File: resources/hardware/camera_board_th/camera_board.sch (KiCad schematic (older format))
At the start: 10 parts, among them P1 CONN_01X03, Q1 Q_NPN_EBC

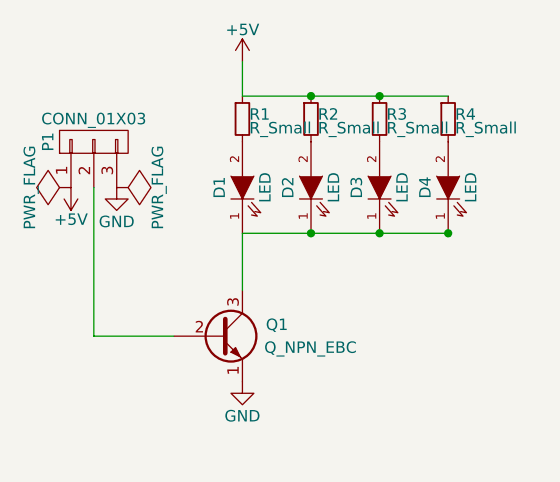
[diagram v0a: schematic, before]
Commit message: nt
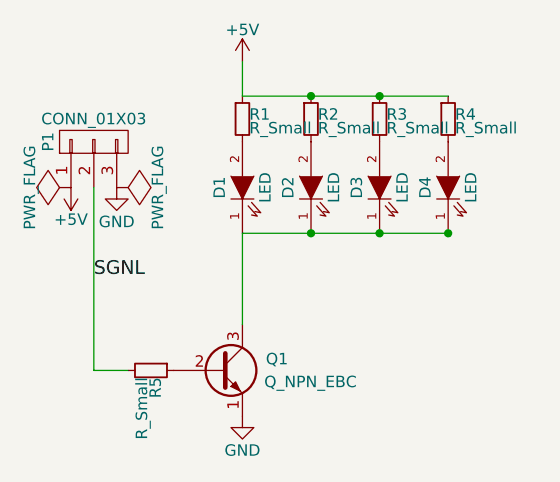
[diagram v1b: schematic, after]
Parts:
- added R5: R_Small, symbol R_Small
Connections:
- net at Q1.2 (B): now also R5.1; no longer P1.2 (P2)
- new net SGNL: P1.2 (P2), R5.2
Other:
- moved on the sheet: Q1
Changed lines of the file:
@@
 L GND #PWR02
 U 1 1 569CFB31
-P 3750 4250
-F 0 "#PWR02" H 3750 4000 50  0001 C CNN
-F 1 "GND" H 3750 4100 50  0000 C CNN
-F 2 "" H 3750 4250 50  0000 C CNN
-F 3 "" H 3750 4250 50  0000 C CNN
-	1    3750 4250
+P 3750 4400
+F 0 "#PWR02" H 3750 4150 50  0001 C CNN
+F 1 "GND" H 3750 4250 50  0000 C CNN
+F 2 "" H 3750 4400 50  0000 C CNN
+F 3 "" H 3750 4400 50  0000 C CNN
+	1    3750 4400
 	1    0    0    -1
 $EndComp
@@
 L Q_NPN_EBC Q1
 U 1 1 56E033A4
-P 3650 4050
-F 0 "Q1" H 3950 4100 50  0000 R CNN
-F 1 "Q_NPN_EBC" H 4250 4000 50  0000 R CNN
-F 2 "" H 3850 4150 50  0000 C CNN
-F 3 "" H 3650 4050 50  0000 C CNN
-	1    3650 4050
+P 3650 4200
+F 0 "Q1" H 3950 4250 50  0000 R CNN
+F 1 "Q_NPN_EBC" H 4250 4150 50  0000 R CNN
+F 2 "" H 3850 4300 50  0000 C CNN
+F 3 "" H 3650 4200 50  0000 C CNN
+	1    3650 4200
 	1    0    0    -1
 $EndComp
@@
 	-1   0    0    1
 $EndComp
-Connection ~ 4050 3600
-Connection ~ 4350 3600
-Wire Wire Line
-	3750 3600 4650 3600
-Connection ~ 4650 3600
-Wire Wire Line
-	3100 3400 3100 4050
-Wire Wire Line
-	3100 4050 3450 4050
 $Comp
 L R_Small R1
@@
 	1    0    0    -1
 $EndComp
+Connection ~ 4050 3600
+Connection ~ 4350 3600
+Wire Wire Line
+	3750 3600 4650 3600
+Connection ~ 4650 3600
 Wire Wire Line
 	3750 3000 4650 3000
@@
 Wire Wire Line
 	3750 2850 3750 3000
+Text Label 3100 3800 0    60   ~ 0
+SGNL
+$Comp
+L R_Small R5
+U 1 1 56E03C9D
+P 3350 4200
+F 0 "R5" H 3380 4220 50  0000 L CNN
+F 1 "R_Small" H 3380 4160 50  0000 L CNN
+F 2 "" H 3350 4200 50  0000 C CNN
+F 3 "" H 3350 4200 50  0000 C CNN
+	1    3350 4200
+	0    1    1    0
+$EndComp
 Wire Wire Line
-	3750 3850 3750 3600
+	3100 3400 3100 4200
+Wire Wire Line
+	3100 4200 3250 4200
+Wire Wire Line
+	3750 4000 3750 3600
 $EndSCHEMATC
